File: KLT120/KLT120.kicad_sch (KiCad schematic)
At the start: 34 parts, among them IC1 LM393BIPWR, IC2 LM393BIPWR, Q1 2N7002K, Q2 2N7002K

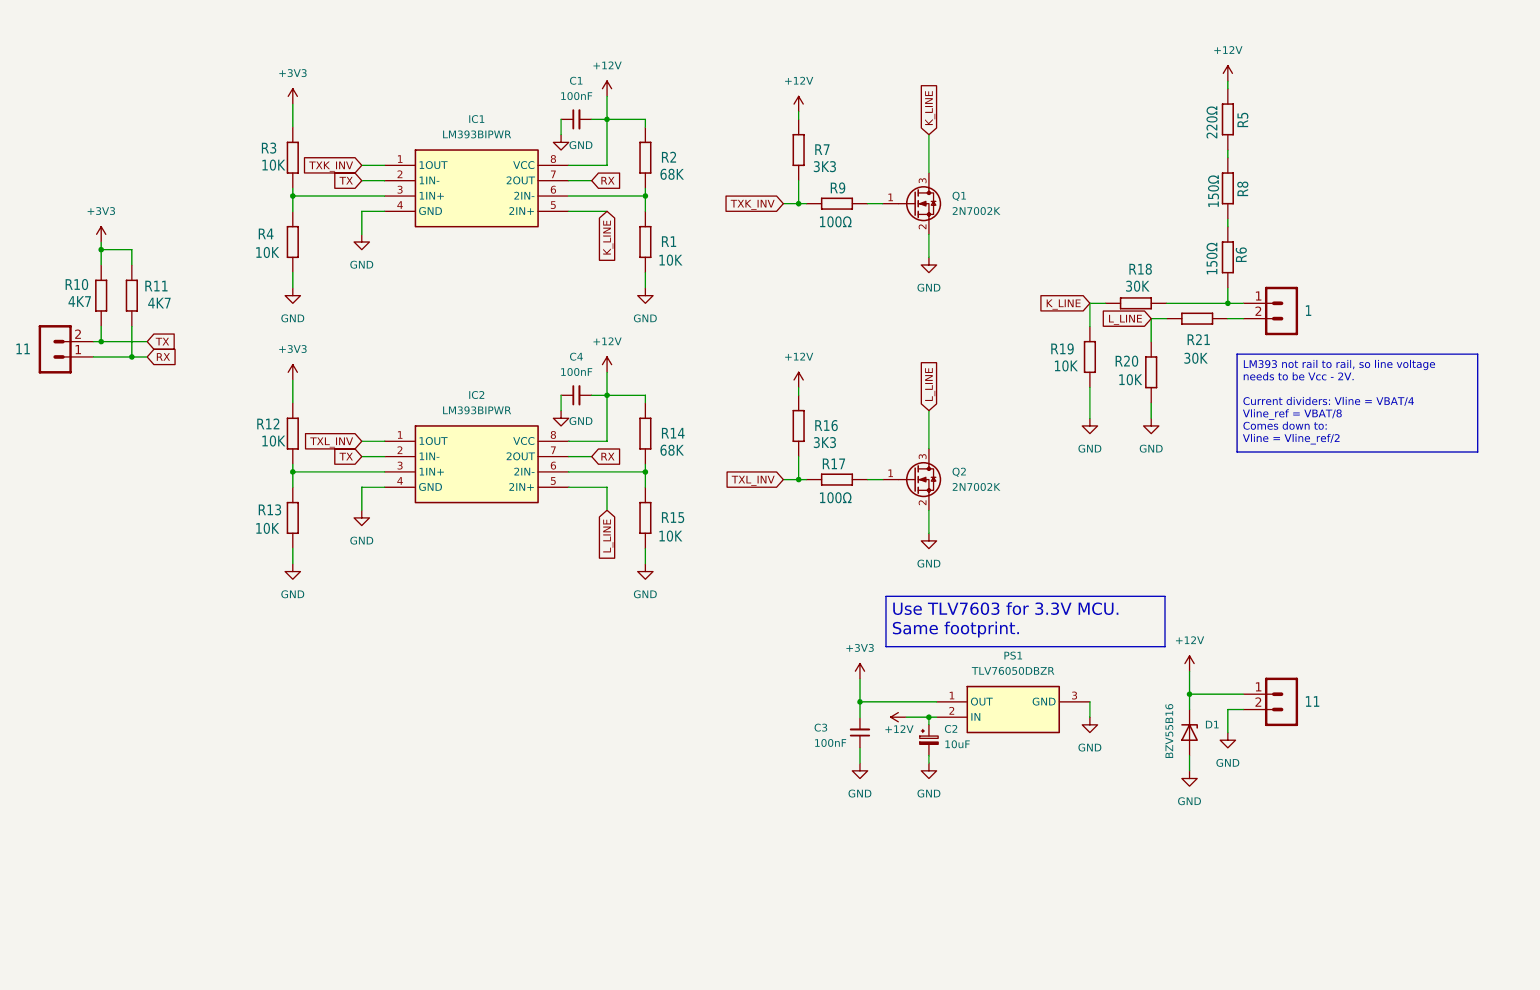
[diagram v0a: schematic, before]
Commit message: v0.11
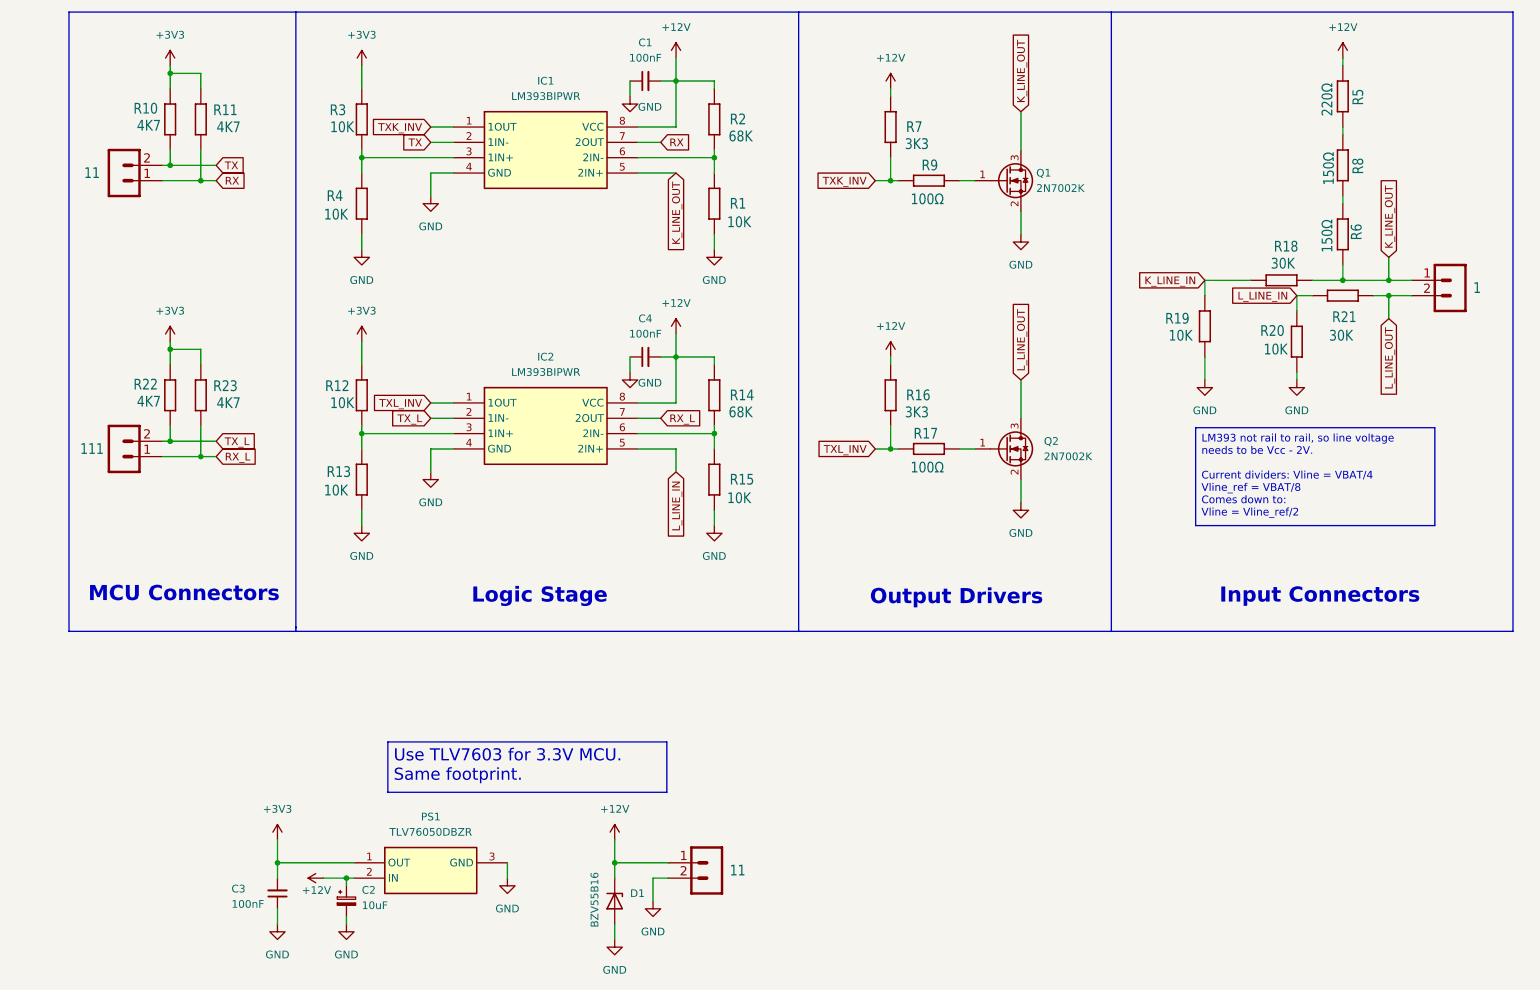
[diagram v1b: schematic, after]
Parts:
- added 111: (no value), 3_pins:90-2, symbol 3_pins:TERMINAL_2PINS
- added R22, R23: 4K7, cap_mult_pins:M0805, symbol cap_mult_pins:R-EU_M0805
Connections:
- net +3V3: now also R22.2, R23.2
- net RX: no longer IC2.7 (2OUT)
- net TX: no longer IC2.2 (1IN-)
- net L_LINE_OUT: now reaches 1.2, R21.1
- net L_LINE_OUT: now also Q2.3 (D)
- net K_LINE_OUT: now reaches 1.1, R18.1, R6.1
- net K_LINE_OUT: now also IC1.5 (2IN+), Q1.3 (D)
- net K_LINE renamed K_LINE_IN
- net K_LINE_IN: no longer IC1.5 (2IN+), Q1.3 (D)
- net L_LINE renamed L_LINE_IN
- net L_LINE_IN: no longer Q2.3 (D)
- new net RX_L: 111.1, IC2.7 (2OUT), R23.1
- new net TX_L: 111.2, IC2.2 (1IN-), R22.1
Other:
- note added: "Input Connectors"
- note added: "Logic Stage"
- note added: "MCU Connectors"
- note added: "Output Drivers"
- company: (none) -> Standalone K/L Line Transceiver for 5/3.3V MCUs
- title: (none) -> KLT120
- moved on the sheet: 1, 11, C1, C2, C3, C4, D1, IC1, IC2, PS1, Q1, Q2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
